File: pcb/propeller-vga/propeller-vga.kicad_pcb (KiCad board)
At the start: 2 copper layers, 125.7 x 53.3 mm, 36 parts, among them J1 USB_A, J2 PPRG, J3 SER, J4 VGA, SW1 SW_Push, U1 P8X32A-D40, U2 24LC256, U3 LD1117S33TR_SOT223, Y1 5MHz

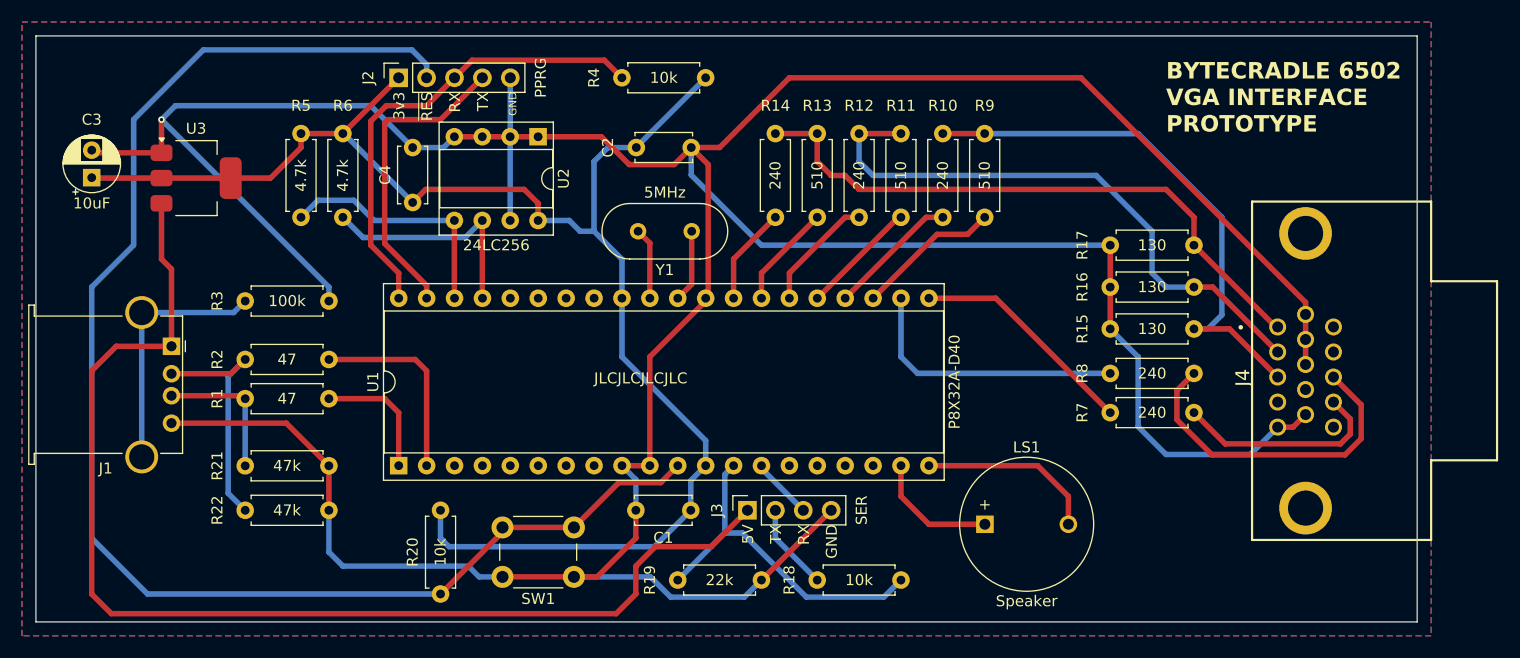
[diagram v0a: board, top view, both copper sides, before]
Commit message: Updating schematic
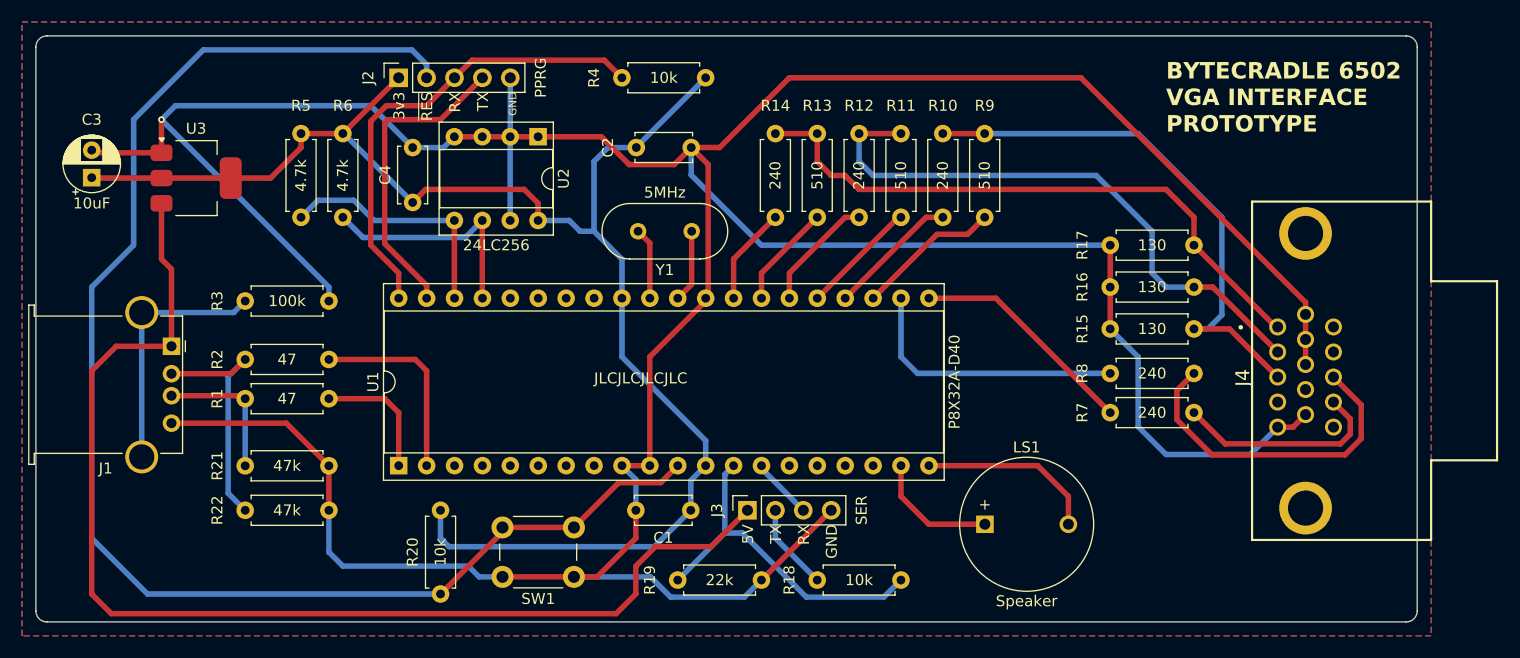
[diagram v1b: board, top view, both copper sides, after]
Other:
- outline, holes or cut-outs redrawn
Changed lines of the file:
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@@
 	)
 	(paper "A4")
+	(title_block
+		(title "Propeller VGA board for ByteCradle 6502 / Prototype")
+		(date "2025-02-08")
+		(rev "0")
+	)
 	(layers
 		(0 "F.Cu" signal)
@@
 		)
 		(property "Value" "240"
-			(at 3.81 0 270)
+			(at 3.81 0 -90)
 			(layer "F.SilkS")
 			(effects
@@
 		)
 		(fp_text user "${REFERENCE}"
-			(at 3.81 0 270)
+			(at 3.81 0 -90)
 			(layer "F.Fab")
 			(effects
@@
 		)
 		(property "Value" "510"
-			(at 3.81 0 270)
+			(at 3.81 0 -90)
 			(layer "F.SilkS")
 			(effects
@@
 		)
 		(fp_text user "${REFERENCE}"
-			(at 3.81 0 270)
+			(at 3.81 0 -90)
 			(layer "F.Fab")
 			(effects
@@
 		)
 		(property "Value" "240"
-			(at 3.81 0 270)
+			(at 3.81 0 -90)
 			(layer "F.SilkS")
 			(effects
@@
 		)
 		(fp_text user "${REFERENCE}"
-			(at 3.81 0 270)
+			(at 3.81 0 -90)
 			(layer "F.Fab")
 			(effects
@@
 		)
 		(property "Value" "510"
-			(at 3.81 0 270)
+			(at 3.81 0 -90)
 			(layer "F.SilkS")
 			(effects
@@
 		)
 		(fp_text user "${REFERENCE}"
-			(at 3.81 0 270)
+			(at 3.81 0 -90)
 			(layer "F.Fab")
 			(effects
@@
 		(tags "C Disc series Radial pin pitch 5.00mm  diameter 5mm width 2.5mm Capacitor")
 		(property "Reference" "C4"
-			(at 2.5 -2.5 270)
+			(at 2.5 -2.5 -90)
 			(layer "F.SilkS")
 			(effects
@@
 		)
 		(property "Value" "C"
-			(at 2.5 2.5 270)
+			(at 2.5 2.5 -90)
 			(layer "F.Fab")
 			(effects
@@
 		)
 		(fp_text user "${REFERENCE}"
-			(at 2.5 0 270)
+			(at 2.5 0 -90)
 			(layer "F.Fab")
 			(effects
@@
 		(tags "Through hole socket strip THT 1x04 2.54mm single row")
 		(property "Reference" "J3"
-			(at 0 -2.77 270)
+			(at 0 -2.77 -90)
 			(layer "F.SilkS")
 			(effects
@@
 		)
 		(property "Value" "SER"
-			(at 0 10.39 270)
+			(at 0 10.39 -90)
 			(layer "F.SilkS")
 			(effects
@@
 		)
 		(fp_text user "${REFERENCE}"
-			(at 0 3.81 360)
+			(at 0 3.81 0)
 			(layer "F.Fab")
 			(effects
@@
 		)
 		(property "Value" "510"
-			(at 3.81 0 270)
+			(at 3.81 0 -90)
 			(layer "F.SilkS")
 			(effects
@@
 		)
 		(fp_text user "${REFERENCE}"
-			(at 3.81 0 270)
+			(at 3.81 0 -90)
 			(layer "F.Fab")
 			(effects
@@
 		)
 		(fp_text user "${REFERENCE}"
-			(at 1.25 0 270)
+			(at 1.25 0 -90)
 			(layer "F.Fab")
 			(effects
@@
 		(tags "Through hole socket strip THT 1x05 2.54mm single row")
 		(property "Reference" "J2"
-			(at 0 -2.77 270)
+			(at 0 -2.77 -90)
 			(layer "F.SilkS")
 			(effects
@@
 		)
 		(property "Value" "PPRG"
-			(at 0 12.93 270)
+			(at 0 12.93 -90)
 			(layer "F.SilkS")
 			(effects
@@
 		)
 		(fp_text user "${REFERENCE}"
-			(at 0 5.08 360)
+			(at 0 5.08 0)
 			(layer "F.Fab")
 			(effects
@@
 		(tags "Connector")
 		(property "Reference" "J4"
-			(at -0.635 -17.145 270)
+			(at -0.635 -17.145 -90)
 			(layer "F.SilkS")
 			(effects
@@
 		)
 		(property "Value" "VGA"
-			(at -0.3681 -3.83652 270)
+			(at -0.3681 -3.83652 -90)
 			(layer "F.SilkS")
 			(hide yes)
@@
 		)
 		(fp_text user "${REFERENCE}"
-			(at -0.3681 -3.83652 270)
+			(at -0.3681 -3.83652 -90)
 			(layer "F.Fab")
 			(effects
@@
 		)
 		(property "Value" "240"
-			(at 3.81 0 270)
+			(at 3.81 0 -90)
 			(layer "F.SilkS")
 			(effects
@@
 		)
 		(fp_text user "${REFERENCE}"
-			(at 3.81 0 270)
+			(at 3.81 0 -90)
 			(layer "F.Fab")
 			(effects
@@
 		)
 	)
-	(gr_rect
-		(start 105.41 40.64)
-		(end 231.14 93.98)
+	(gr_arc
+		(start 106.41 93.98)
+		(mid 105.702893 93.687107)
+		(end 105.41 92.98)
+		(stroke
+			(width 0.05)
+			(type default)
+		)
+		(layer "Edge.Cuts")
+	)
+	(gr_line
+		(start 105.41 92.98)
+		(end 105.41 41.64)
+		(stroke
+			(width 0.05)
+			(type default)
+		)
+		(layer "Edge.Cuts")
+	)
+	(gr_line
+		(start 231.14 41.64)
+		(end 231.14 92.98)
+		(stroke
+			(width 0.05)
+			(type default)
+		)
+		(layer "Edge.Cuts")
+	)
+	(gr_arc
+		(start 230.14 40.64)
+		(mid 230.847107 40.932893)
+		(end 231.14 41.64)
+		(stroke
+			(width 0.05)
+			(type default)
+		)
+		(layer "Edge.Cuts")
+	)
+	(gr_line
+		(start 230.14 93.98)
+		(end 106.41 93.98)
+		(stroke
+			(width 0.05)
+			(type default)
+		)
+		(layer "Edge.Cuts")
+	)
+	(gr_arc
+		(start 105.41 41.64)
+		(mid 105.702893 40.932893)
+		(end 106.41 40.64)
+		(stroke
+			(width 0.05)
+			(type default)
+		)
+		(layer "Edge.Cuts")
+	)
+	(gr_line
+		(start 106.41 40.64)
+		(end 230.14 40.64)
+		(stroke
+			(width 0.05)
+			(type default)
+		)
+		(layer "Edge.Cuts")
+	)
+	(gr_arc
+		(start 231.14 92.98)
+		(mid 230.847107 93.687107)
+		(end 230.14 93.98)
 		(stroke
 			(width 0.05)
 			(type default)
 		)
-		(fill none)
 		(layer "Edge.Cuts")
 	)
